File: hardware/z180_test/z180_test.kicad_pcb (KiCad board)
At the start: 2 copper layers, 48 parts, among them J1 Conn_01x04, J2 DIN41612_02x32_AB, J3 Conn_01x04, J4 Conn_01x06, J5 Conn_01x06, J6 Conn_02x17_Counter_Clockwise, SW1 SW_Push, U1 74AHC32, U10 8255A, U11 28C256, U12 AS6C4008-55PCN, U2 74LS244, U3 74LS244, U4 74LS244, U5 74LS245, U6 Z180, U7 74HC04, U8 74LS139, U9 74HC14, X1 OSC 12.288MHz 5V

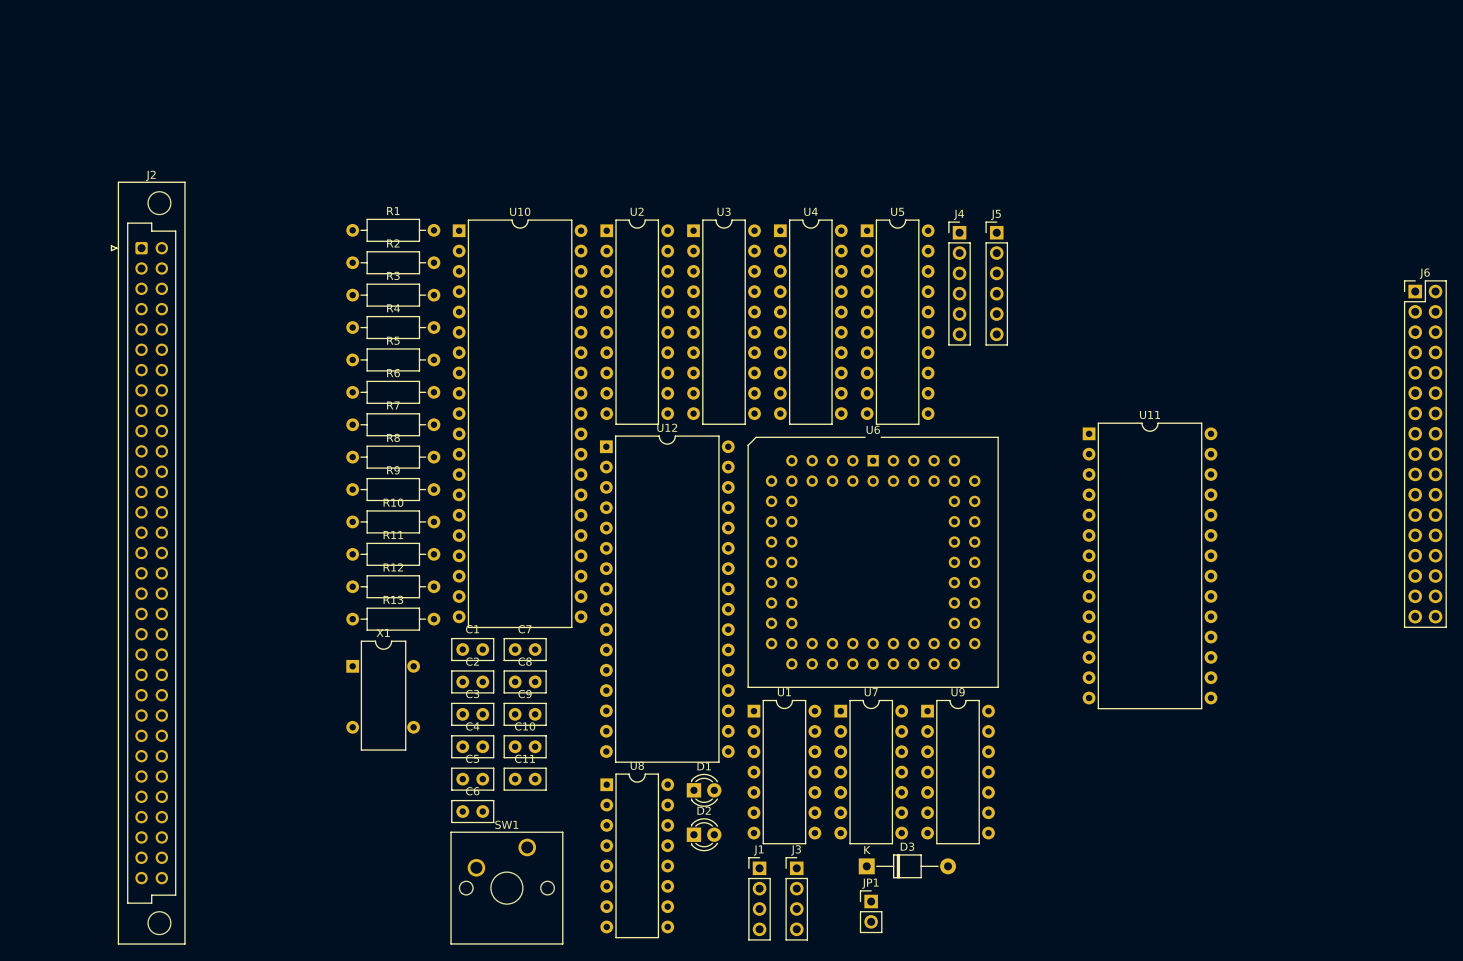
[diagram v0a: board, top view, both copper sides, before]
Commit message: tentative placement
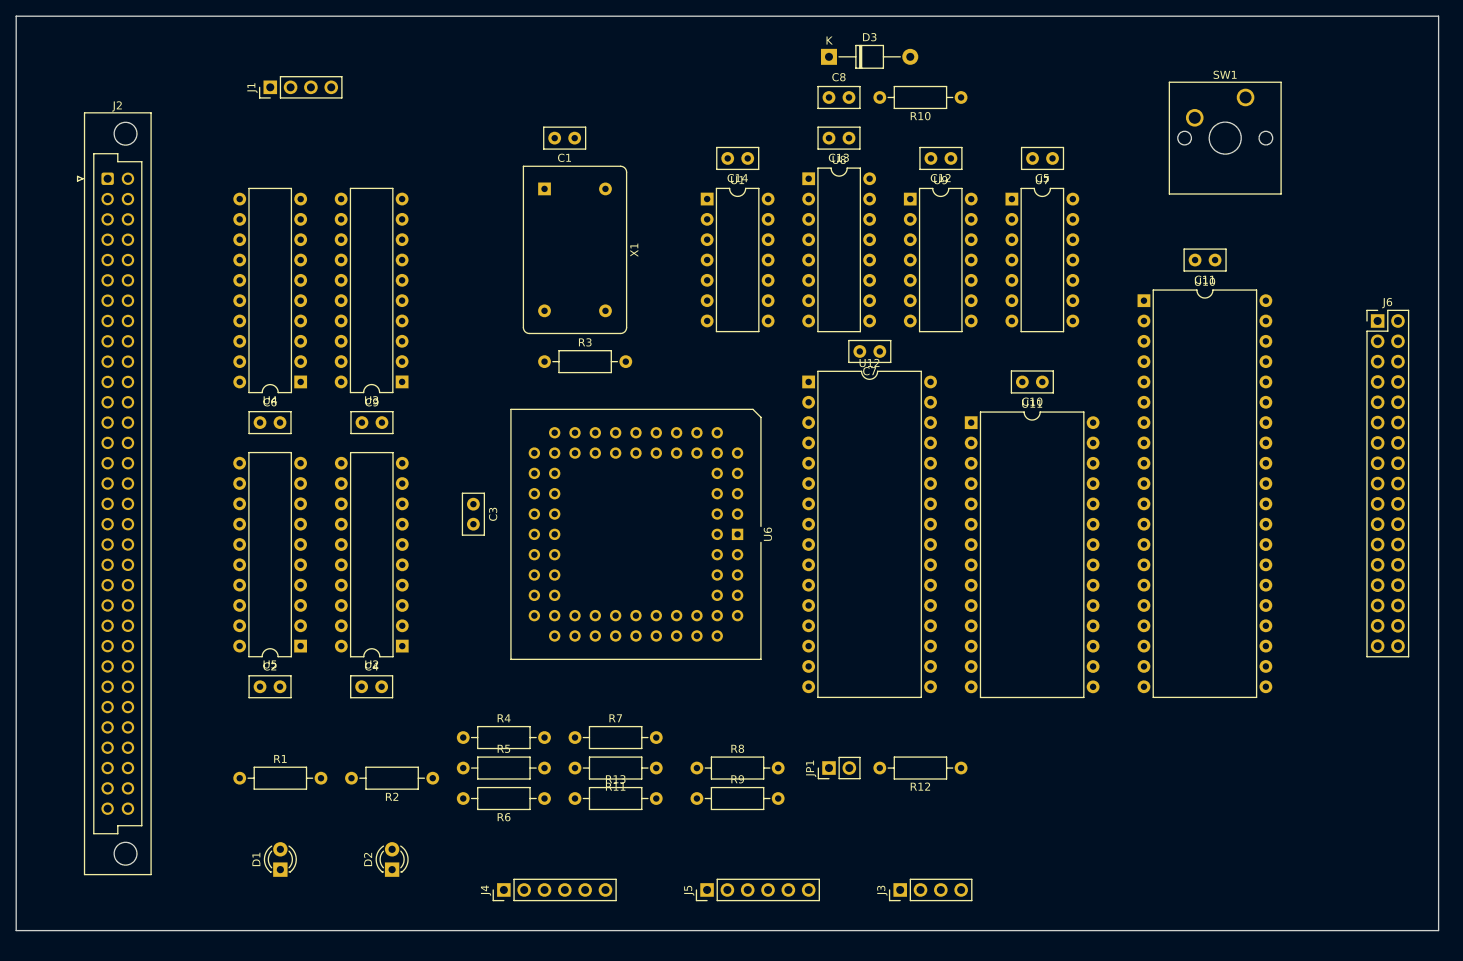
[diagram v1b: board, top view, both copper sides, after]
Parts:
- added C12: .01uF, Capacitor_THT:C_Disc_D5.0mm_W2.5mm_P2.50mm, F.Cu at (144.8, 45.7)
- added C13: .01uF, Capacitor_THT:C_Disc_D5.0mm_W2.5mm_P2.50mm, F.Cu at (132.0, 43.2)
- added C14: .01uF, Capacitor_THT:C_Disc_D5.0mm_W2.5mm_P2.50mm, F.Cu at (119.4, 45.7)
- X1: value OSC 12.288MHz 5V -> ACO-xxxMHz-A; footprint Oscillator:Oscillator_SeikoEpson_SG-8002DC -> Oscillator:Oscillator_DIP-14
- moved SW1 129.8 mm to (181.6, 38.1)
- moved J1 115.2 mm to (59.7, 36.8), turned to 90 degrees
- moved C11 108.9 mm to (177.8, 58.4), turned to 180 degrees
- moved C5 107.0 mm to (157.5, 45.7), turned to 180 degrees
- moved D3 101.3 mm to (129.5, 33.0)
- moved J4 100.0 mm to (88.9, 137.2), turned to 90 degrees
- moved R10 92.7 mm to (146.1, 38.1), turned to 180 degrees
- moved J5 89.8 mm to (114.3, 137.2), turned to 90 degrees
- moved U5 87.8 mm to (63.5, 106.7), turned to 180 degrees
- moved U10 86.0 mm to (168.9, 63.5)
- moved C8 82.9 mm to (129.5, 38.1)
- moved C10 80.1 mm to (156.2, 73.7), turned to 180 degrees
- moved U8 79.8 mm to (127.0, 48.3)
- moved R12 79.4 mm to (146.1, 121.9), turned to 180 degrees
- moved R1 69.9 mm to (55.9, 123.2)
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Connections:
- X1 pad 8: VCC -> Net-(U6-EXTAL)
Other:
- board outline added: 177.8 x 114.3 mm
